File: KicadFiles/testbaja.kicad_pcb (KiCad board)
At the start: 2 copper layers, 158.8 x 144.8 mm, 10 parts, among them J1 Conn_01x05_Male, J2 Conn_01x08_Female, J3 Conn_01x04_Female, J4 Conn_01x04_Female, J5 Conn_01x16_Female, J6 Conn_01x04_Female, J7 Conn_01x04_Female, J8 Conn_01x04_Female, J9 Conn_01x30_Female

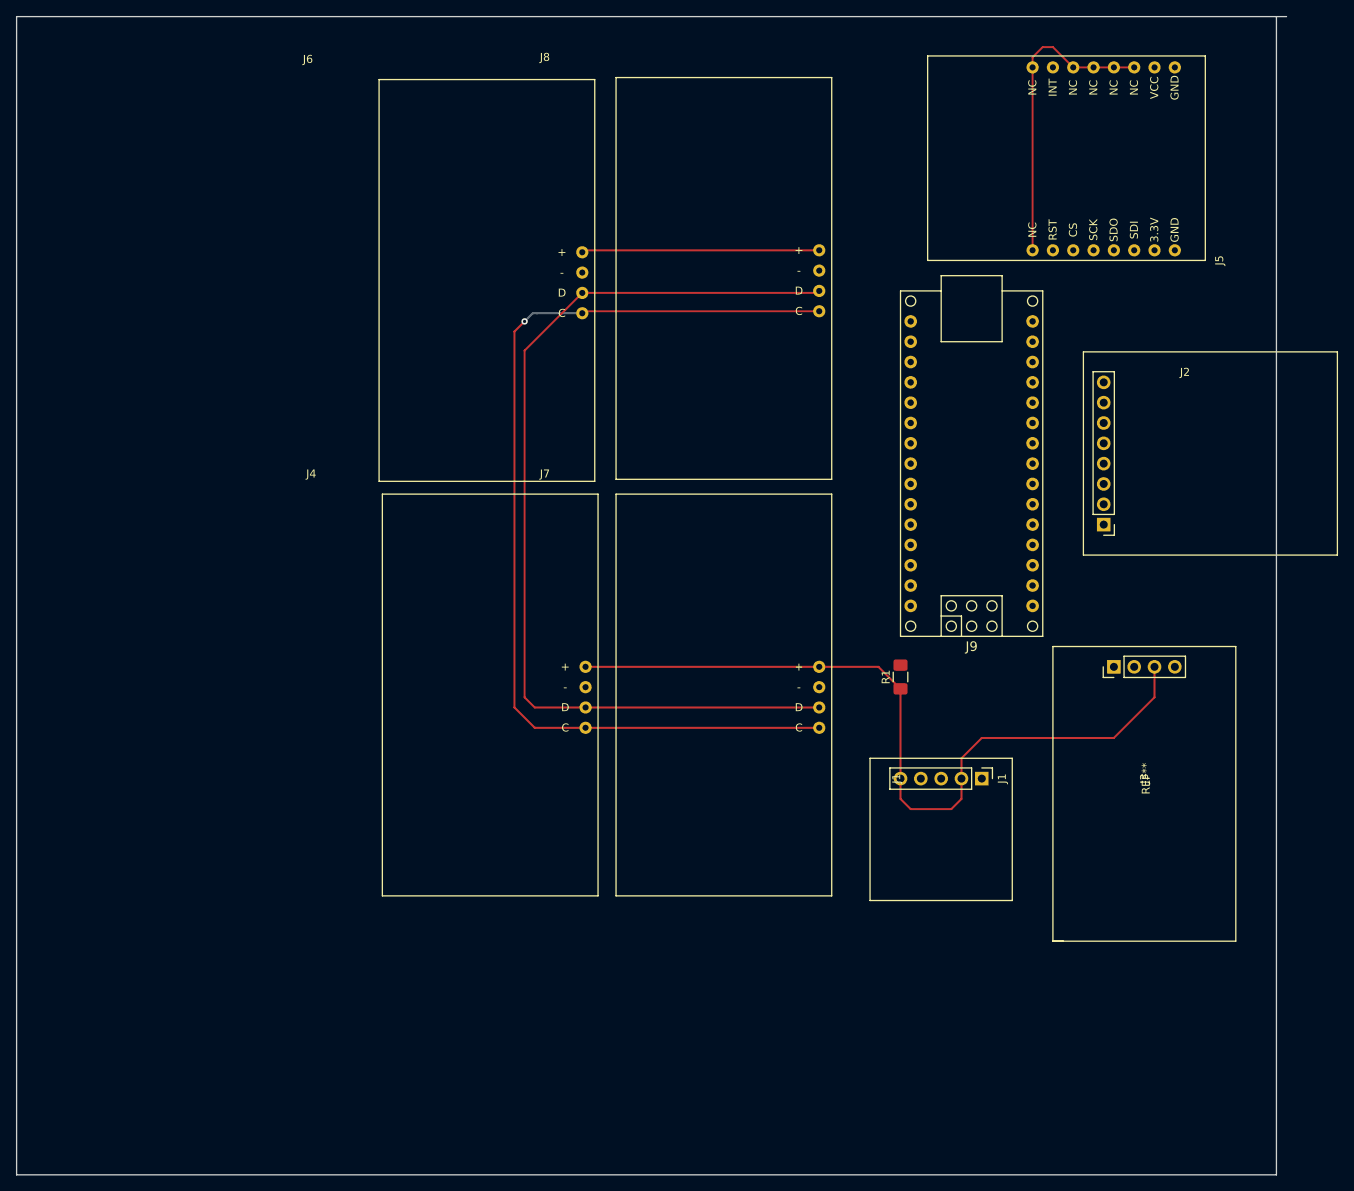
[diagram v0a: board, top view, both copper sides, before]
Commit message: all routed
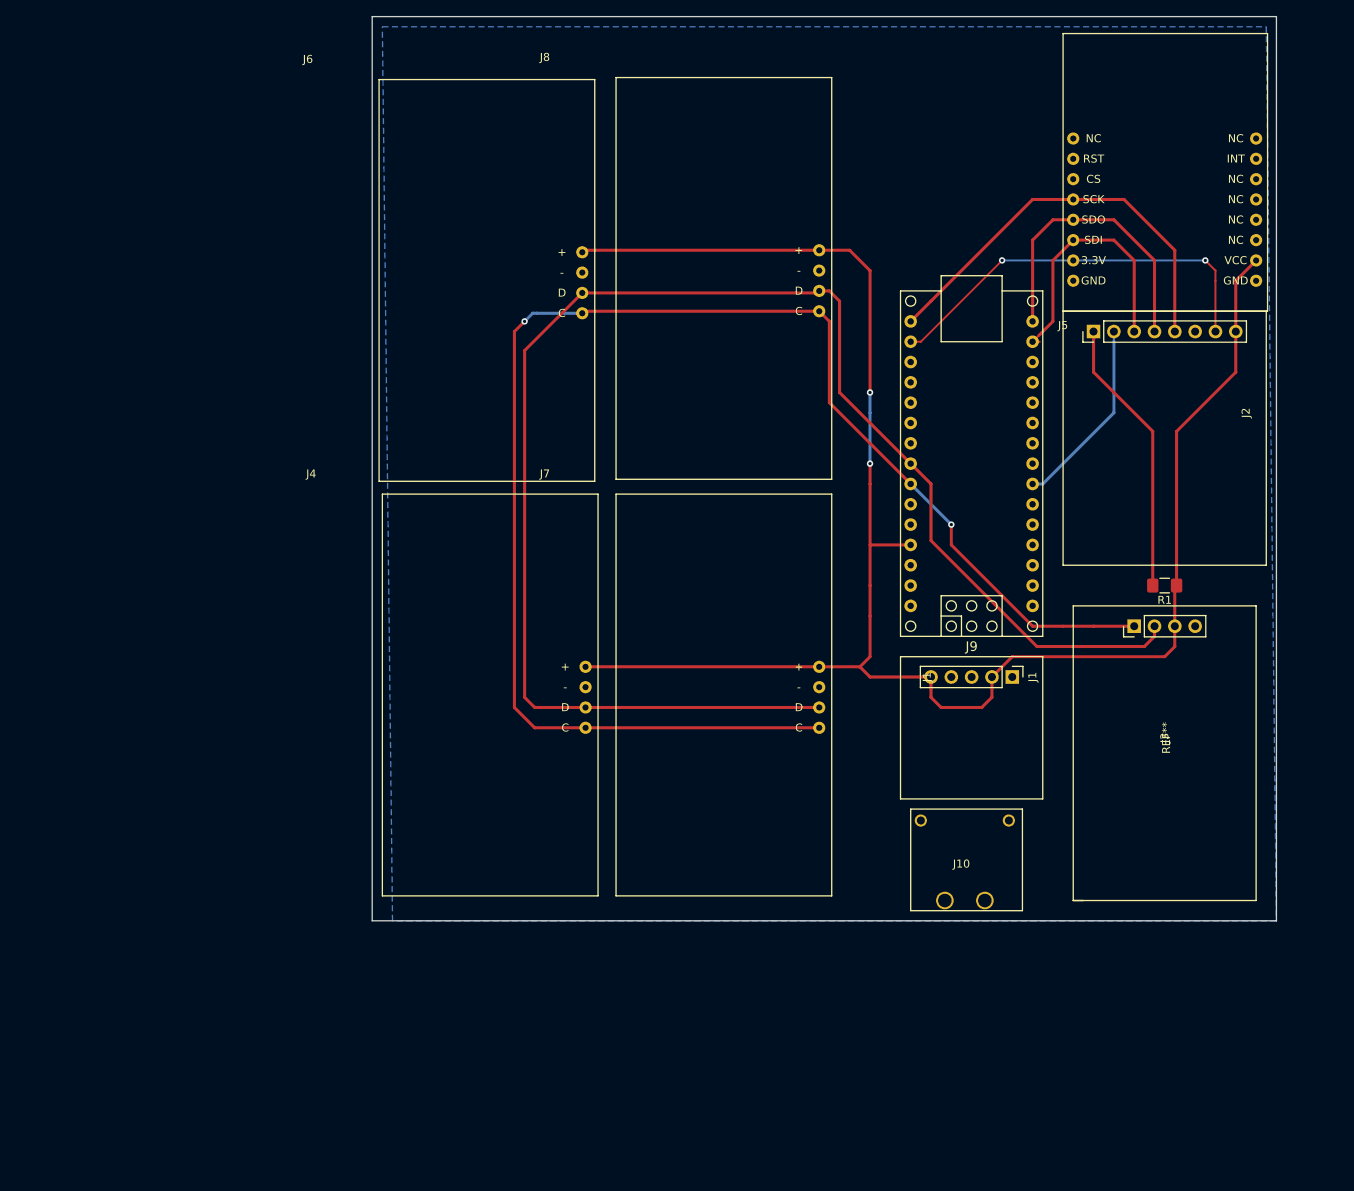
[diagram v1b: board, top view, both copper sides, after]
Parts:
- added J10: Conn_01x04_Female, TestBaja:DC_Connector, F.Cu at (147.3, 133.3)
- moved R1 34.9 mm to (177.8, 94.0), turned to 180 degrees
- moved J5 18.9 mm to (165.1, 59.7), turned to 0 degrees
- moved J2 17.7 mm to (186.7, 62.2), turned to 90 degrees
- moved J1 13.3 mm to (158.8, 105.4)
- moved J3 5.68 mm to (177.8, 99.1)
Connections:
- J2 pad 5: /CLK -> /SCK
- J5 pad 2: /3v3 -> /3V3
- J9 pad 17: /3v3 -> /3V3
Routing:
- net /5V: track 128.8 -> 226.6 mm, vias 0 -> 2
- net /SDA: track 120.6 -> 193.6 mm
- net /SCL: track 125.3 -> 188.4 mm, vias 1 -> 2
- net /SCK: track 0.00 -> 52.1 mm
- net /3V3: track 0.00 -> 50.5 mm, vias 0 -> 2
- net /NC: track 38.4 -> 0.00 mm
- net /d12: track 0.00 -> 37.4 mm
- net /CD: track 0.00 -> 34.8 mm
- net /d11: track 0.00 -> 33.3 mm
- net /d4: track 0.00 -> 24.0 mm
- added copper zone on B.Cu, net /GND
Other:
- board size 158.8 x 144.8 mm -> 113 x 113 mm

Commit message: ORDERED BOARDS
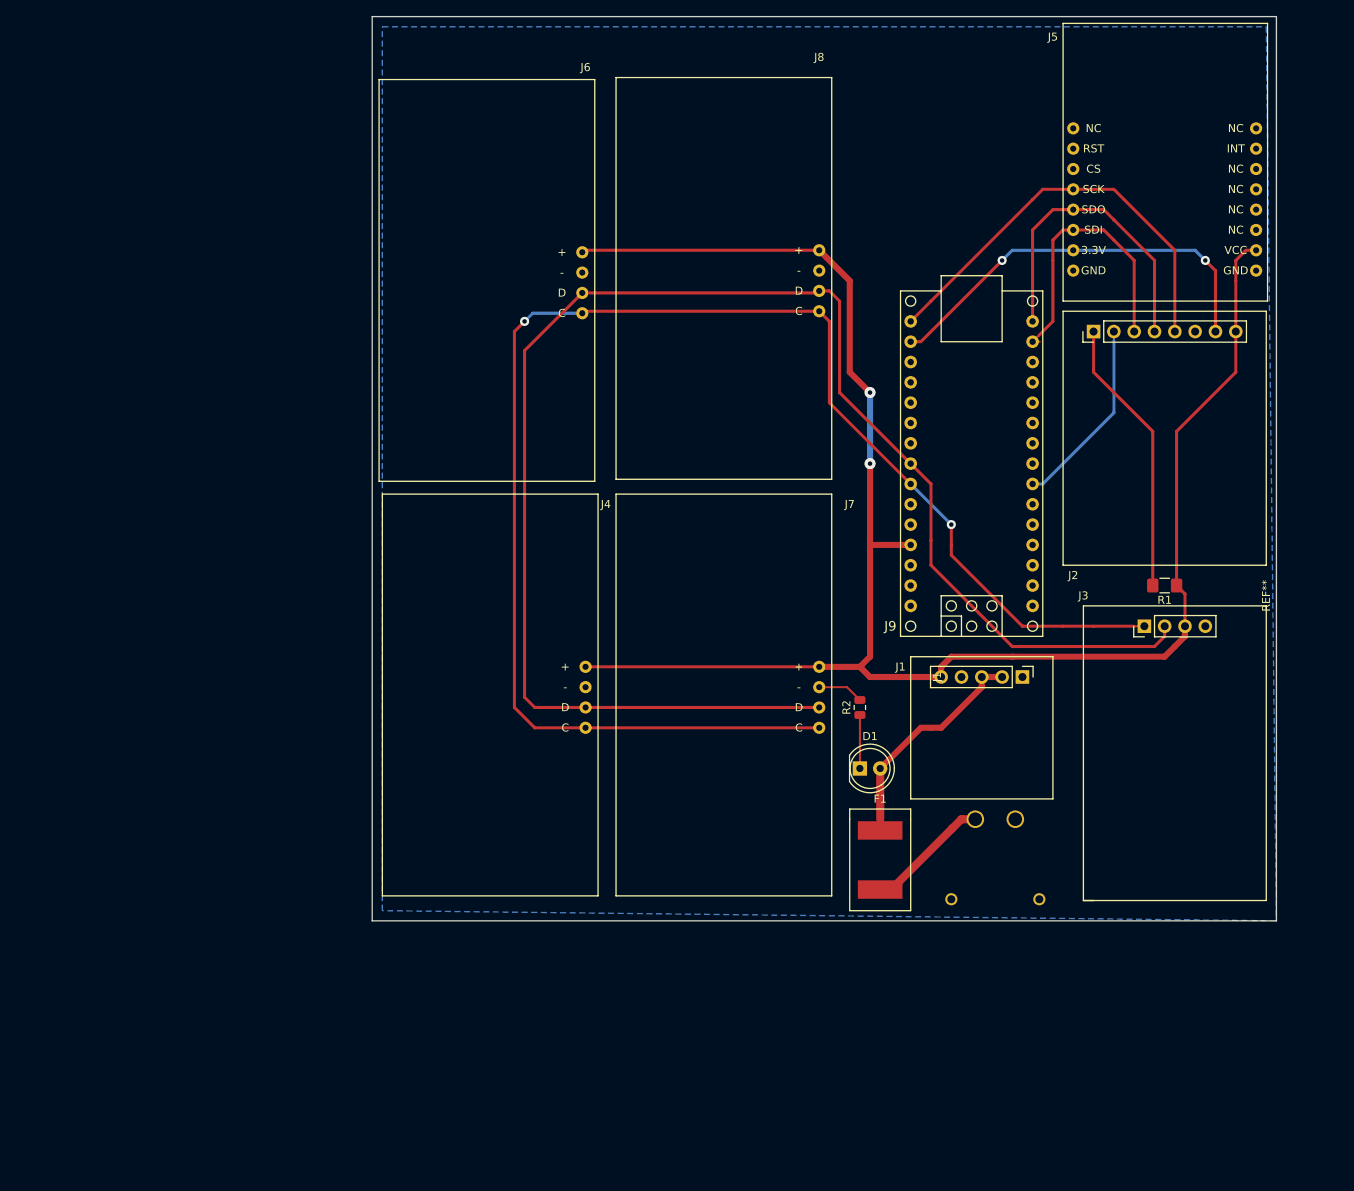
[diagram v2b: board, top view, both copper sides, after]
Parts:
- added D1: RED, LED_THT:LED_D5.0mm_FlatTop, F.Cu at (139.7, 116.8)
- added F1: Fuse, TestBaja:Fuse_0ZCFSeries, F.Cu at (142.2, 125.7)
- added R2: 220, Resistor_SMD:R_0805_2012Metric, F.Cu at (139.7, 109.2)
- J10: moved to B.Cu
- moved J10 10.9 mm to (151.1, 123.2)
- moved J1 1.27 mm to (160.0, 105.4)
- moved J5 1.27 mm to (165.1, 58.4)
- moved J3 1.27 mm to (179.1, 99.1)
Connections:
- J1 pad 2: /5V -> /IN
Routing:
- net /IN: track 0.00 -> 28.5 mm
- net /IN_UNFUSED: track 0.00 -> 15.9 mm
- net Net-(D1-Pad1): track 0.00 -> 6.68 mm
- net /GND: track 0.00 -> 5.74 mm
- net /5V: track 226.6 -> 222.2 mm
- net /SDA: track 193.6 -> 197.4 mm
- net /d11: track 33.3 -> 35.8 mm
- net /SCL: track 188.4 -> 190.4 mm
- net /d12: track 37.4 -> 39.2 mm
- net /3V3: track 50.5 -> 51.5 mm
- net /SCK: track 52.1 -> 53.2 mm
